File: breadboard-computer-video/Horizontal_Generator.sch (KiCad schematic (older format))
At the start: 3 parts

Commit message: Finished H and V generators
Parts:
- added U? (x4): 74LS21, symbol 74xx:74LS21
- added U? (x4): 74LS32, symbol 74xx:74LS32
- added U? (x4): 74LS04, symbol 74xx:74LS04
- added U?: 74LS08, symbol 74xx:74LS08
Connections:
- net labels added: H_Blank, H_Sync
- wire segments 5 -> 59

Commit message: Finished sync generation, added pixel clock
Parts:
- removed U? (x3): 74LS168, symbol 74xx:74LS168
- added U? (x3): 74LS161, symbol 74xx:74LS161
- added U?: 74LS30, symbol 74xx:74LS30
- added U? (x2): 74LS04, symbol 74xx:74LS04
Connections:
- net labels added: LINE
- wire segments 59 -> 130

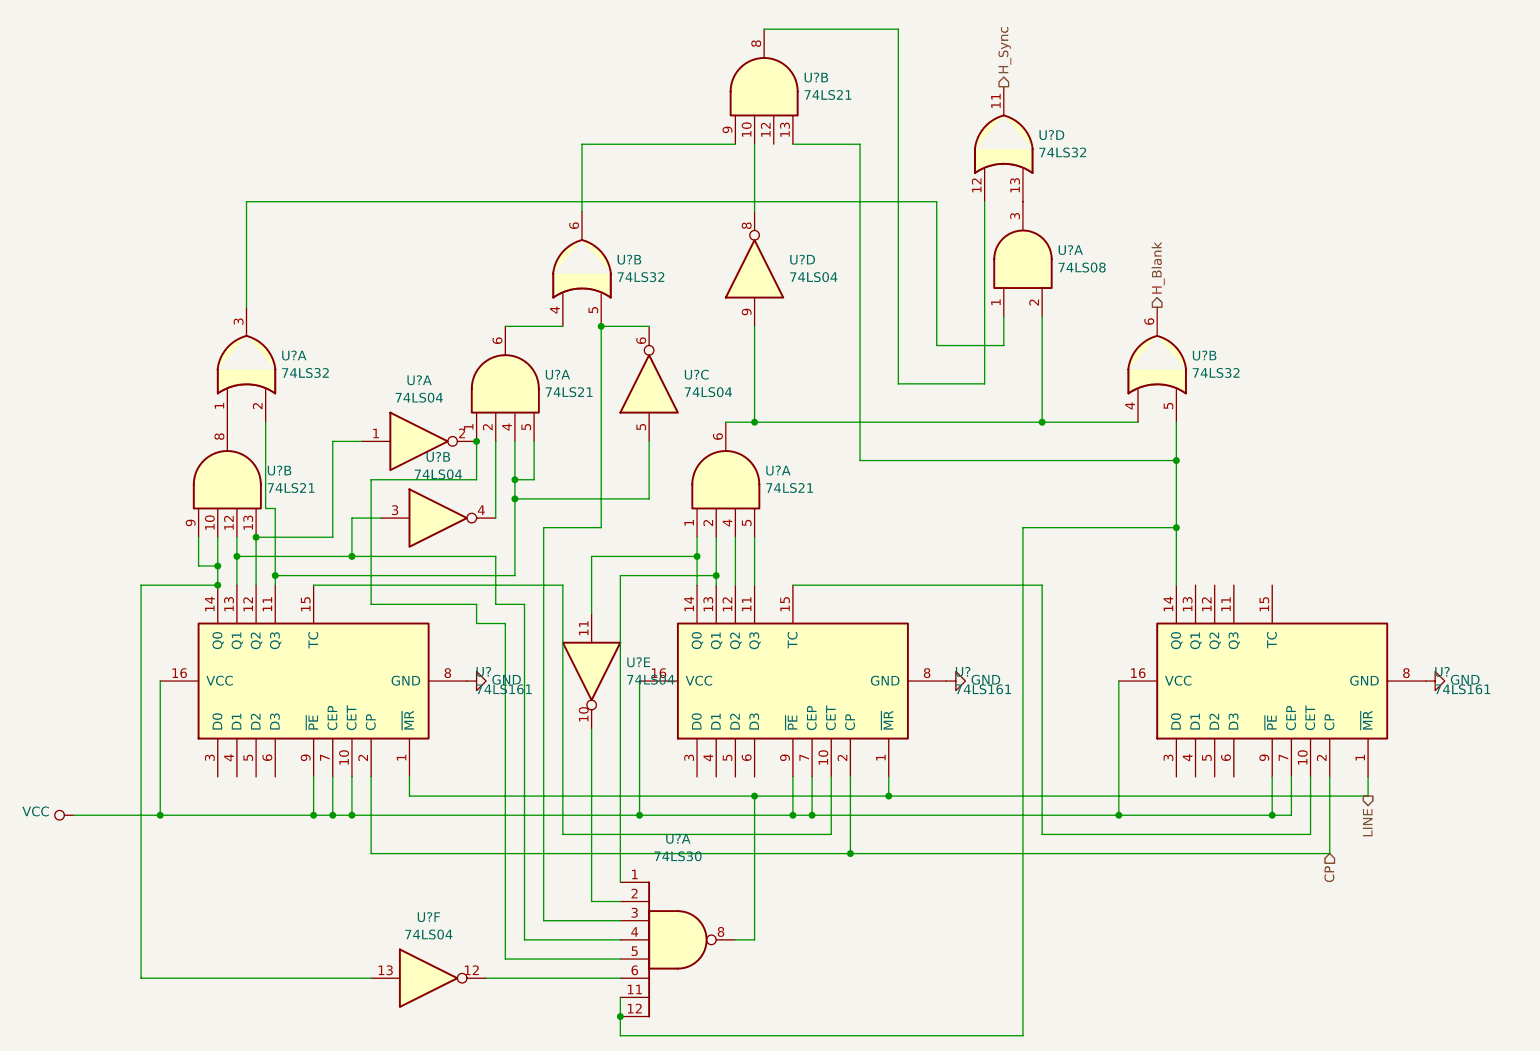
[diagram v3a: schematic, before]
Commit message: finished
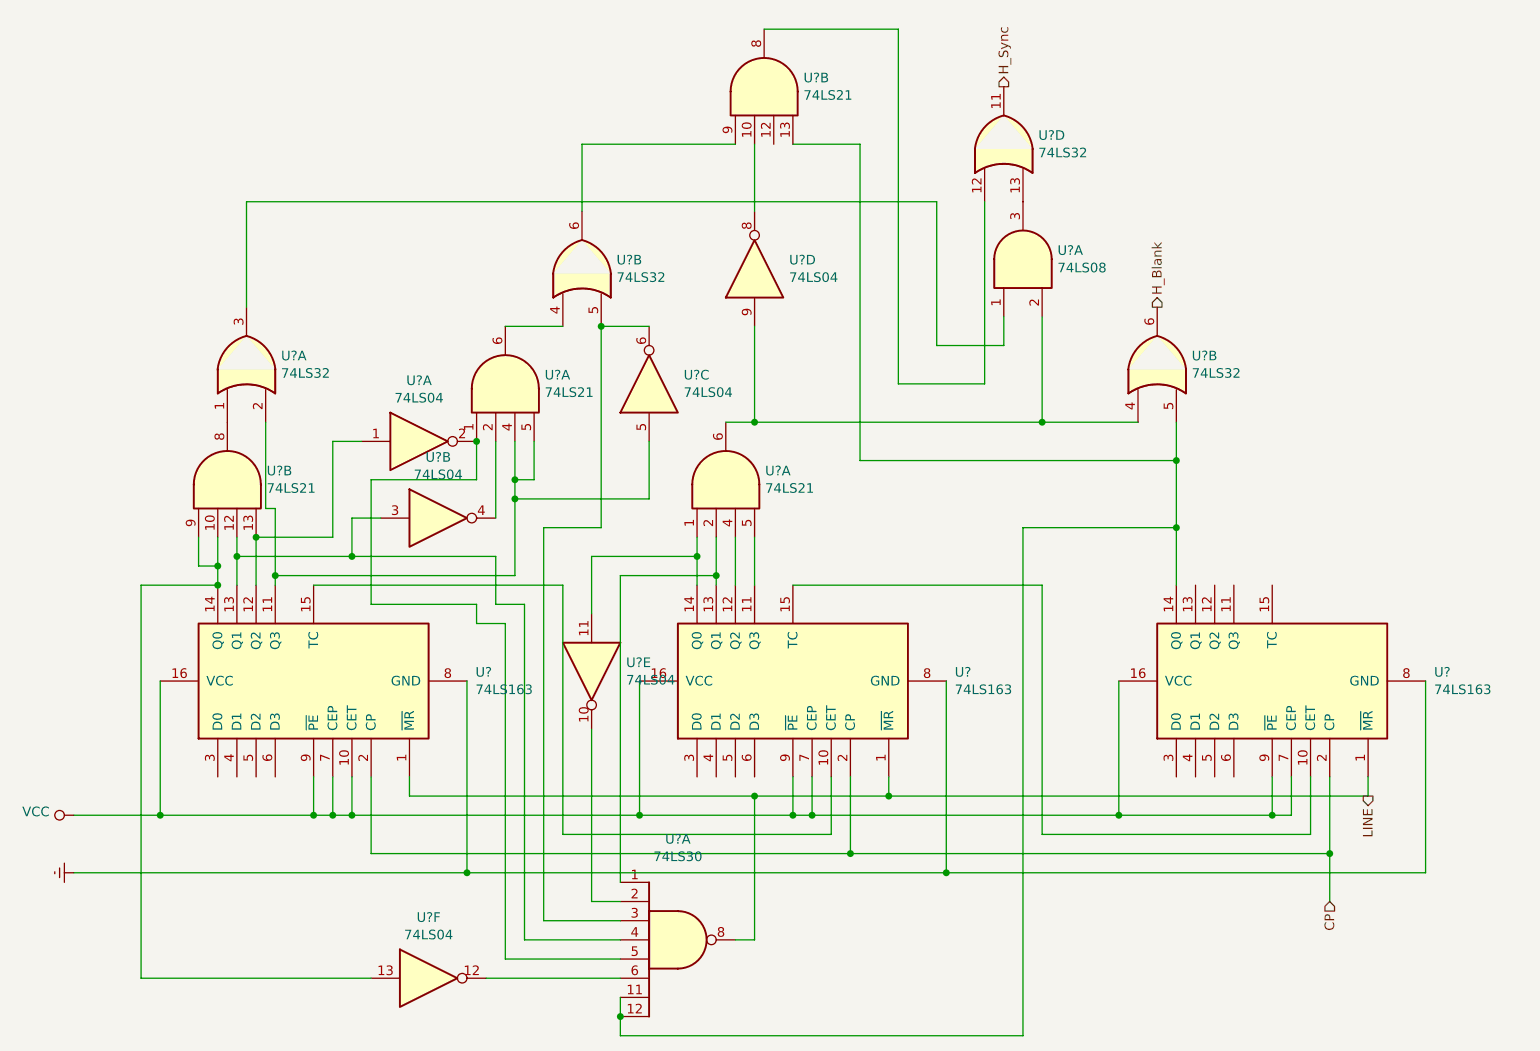
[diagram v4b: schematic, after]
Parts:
- removed U? (x3): 74LS161, symbol 74xx:74LS161
- added U? (x3): 74LS163, symbol 74xx:74LS163
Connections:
- net CP: now also U?.2 (CP), U?.2 (CP), U?.2 (CP)
- net LINE: now also U?.1 (~MR), U?.1 (~MR), U?.1 (~MR)
- net VCC: now also U?.10 (CET), U?.16 (VCC), U?.16 (VCC), U?.16 (VCC), U?.7 (CEP), U?.7 (CEP), U?.7 (CEP), U?.9 (~PE), U?.9 (~PE), U?.9 (~PE)
- net at U?.1, U?.11: now also U?.14 (Q0)
- net at U?.1, U?.2: now also U?.13 (Q1)
- net at U?.4: now also U?.12 (Q2)
- net at U?.5: now also U?.11 (Q3)
- net at U?.10, U?.13, U?.9: now also U?.14 (Q0)
- net at U?.12, U?.3, U?.4: now also U?.13 (Q1)
- net at U?.1, U?.13: now also U?.12 (Q2)
- net at U?.2, U?.4, U?.5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: now also U?.11 (Q3)
- net at U?.11, U?.12, U?.13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: now also U?.14 (Q0)
- new net: U?.10 (CET), U?.15 (TC) (x2)
- new net Earth: U?.8 (GND), U?.8 (GND), U?.8 (GND)
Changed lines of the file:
@@
 $Descr A4 11693 8268
 encoding utf-8
-Sheet 3 4
+Sheet 3 5
 Title ""
 Date ""
@@
 Comment4 ""
 $EndDescr
-Text HLabel 8350 6050 3    50   Input ~ 0
+Text HLabel 8350 6300 3    50   Input ~ 0
 CP
 Wire Wire Line
 	3350 5650 3350 6050
-$Comp
-L power:GND #PWR?
-U 1 1 5DBA5B33
-P 6350 5150
-F 0 "#PWR?" H 6350 4900 50  0001 C CNN
-F 1 "GND" V 6355 5022 50  0000 R CNN
-F 2 "" H 6350 5150 50  0001 C CNN
-F 3 "" H 6350 5150 50  0001 C CNN
-	1    6350 5150
-	0    -1   -1   0
-$EndComp
-$Comp
-L power:GND #PWR?
-U 1 1 5DBA5B39
-P 3850 5150
-F 0 "#PWR?" H 3850 4900 50  0001 C CNN
-F 1 "GND" V 3855 5022 50  0000 R CNN
-F 2 "" H 3850 5150 50  0001 C CNN
-F 3 "" H 3850 5150 50  0001 C CNN
-	1    3850 5150
-	0    -1   -1   0
-$EndComp
-$Comp
-L power:GND #PWR?
-U 1 1 5DBAB347
-P 8850 5150
-F 0 "#PWR?" H 8850 4900 50  0001 C CNN
-F 1 "GND" V 8855 5022 50  0000 R CNN
-F 2 "" H 8850 5150 50  0001 C CNN
-F 3 "" H 8850 5150 50  0001 C CNN
-	1    8850 5150
-	0    -1   -1   0
-$EndComp
 Wire Wire Line
 	5850 5650 5850 6050
@@
 Text HLabel 6650 2050 1    50   Output ~ 0
 H_Sync
-$Comp
-L 74xx:74LS161 U?
-U 1 1 5DB5E3FC
-P 5550 5150
-F 0 "U?" V 5596 4306 50  0000 R CNN
-F 1 "74LS161" V 5505 4306 50  0000 R CNN
-F 2 "" H 5550 5150 50  0001 C CNN
-F 3 "http://www.ti.com/lit/gpn/sn74LS161" H 5550 5150 50  0001 C CNN
-	1    5550 5150
-	0    -1   -1   0
-$EndComp
-$Comp
-L 74xx:74LS161 U?
-U 1 1 5DB6099E
-P 3050 5150
-F 0 "U?" V 3096 4306 50  0000 R CNN
-F 1 "74LS161" V 3005 4306 50  0000 R CNN
-F 2 "" H 3050 5150 50  0001 C CNN
-F 3 "http://www.ti.com/lit/gpn/sn74LS161" H 3050 5150 50  0001 C CNN
-	1    3050 5150
-	0    -1   -1   0
-$EndComp
-$Comp
-L 74xx:74LS161 U?
-U 1 1 5DB5CF73
-P 8050 5150
-F 0 "U?" V 8096 4306 50  0000 R CNN
-F 1 "74LS161" V 8005 4306 50  0000 R CNN
-F 2 "" H 8050 5150 50  0001 C CNN
-F 3 "http://www.ti.com/lit/gpn/sn74LS161" H 8050 5150 50  0001 C CNN
-	1    8050 5150
-	0    -1   -1   0
-$EndComp
 Wire Wire Line
 	8350 5650 8350 6050
@@
 Wire Wire Line
 	5350 5750 6050 5750
+$Comp
+L 74xx:74LS163 U?
+U 1 1 5E152224
+P 3050 5150
+F 0 "U?" V 3096 4306 50  0000 R CNN
+F 1 "74LS163" V 3005 4306 50  0000 R CNN
+F 2 "" H 3050 5150 50  0001 C CNN
+F 3 "http://www.ti.com/lit/gpn/sn74LS163" H 3050 5150 50  0001 C CNN
+	1    3050 5150
+	0    -1   -1   0
+$EndComp
+$Comp
+L 74xx:74LS163 U?
+U 1 1 5E1579F5
+P 5550 5150
+F 0 "U?" V 5596 4306 50  0000 R CNN
+F 1 "74LS163" V 5505 4306 50  0000 R CNN
+F 2 "" H 5550 5150 50  0001 C CNN
+F 3 "http://www.ti.com/lit/gpn/sn74LS163" H 5550 5150 50  0001 C CNN
+	1    5550 5150
+	0    -1   -1   0
+$EndComp
+$Comp
+L 74xx:74LS163 U?
+U 1 1 5E15D181
+P 8050 5150
+F 0 "U?" V 8096 4306 50  0000 R CNN
+F 1 "74LS163" V 8005 4306 50  0000 R CNN
+F 2 "" H 8050 5150 50  0001 C CNN
+F 3 "http://www.ti.com/lit/gpn/sn74LS163" H 8050 5150 50  0001 C CNN
+	1    8050 5150
+	0    -1   -1   0
+$EndComp
+Wire Wire Line
+	8850 5150 8850 6150
+Wire Wire Line
+	8850 6150 6350 6150
+Wire Wire Line
+	6350 5150 6350 6150
+Connection ~ 6350 6150
+Wire Wire Line
+	6350 6150 3850 6150
+Wire Wire Line
+	3850 5150 3850 6150
+Connection ~ 3850 6150
+Wire Wire Line
+	3850 6150 1800 6150
+Wire Wire Line
+	8350 6050 8350 6300
+Connection ~ 8350 6050
+$Comp
+L power:Earth #PWR?
+U 1 1 5E1A3868
+P 1800 6150
+F 0 "#PWR?" H 1800 5900 50  0001 C CNN
+F 1 "Earth" H 1800 6000 50  0001 C CNN
+F 2 "" H 1800 6150 50  0001 C CNN
+F 3 "~" H 1800 6150 50  0001 C CNN
+	1    1800 6150
+	0    1    1    0
+$EndComp
 $EndSCHEMATC
